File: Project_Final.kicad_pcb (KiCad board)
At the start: 2 copper layers, 73.5 x 111.5 mm, 54 parts, among them J1 Conn_01x02_Pin, J2 Conn_01x02_Pin, J3 Conn_01x02_Pin, J4 Conn_01x02_Pin, J5 Conn_01x02_Pin, Q1 2N3906, Q10 2N3906, Q11 2N3904, Q12 2N3906, Q13 2N3904, Q14 2N3904, Q15 2N3906, Q16 2N3906, Q17 BSP89, Q18 2N3904, Q19 2N3906, Q2 2N3906, Q20 2N3904, Q21 2N3904, Q22 2N3906, Q3 2N3906, Q4 2N3904, Q5 2N3904, Q6 2N3906, Q7 2N3906, Q8 2N3904, Q9 2N3906

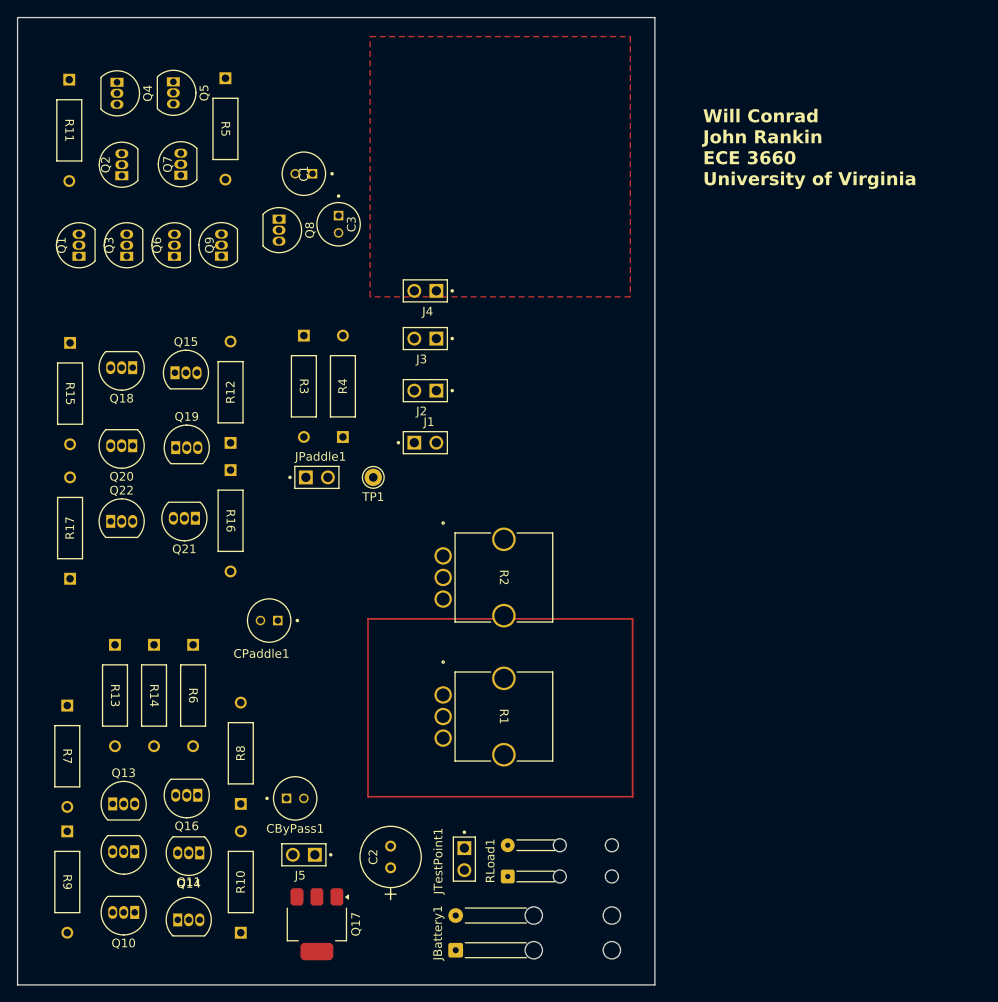
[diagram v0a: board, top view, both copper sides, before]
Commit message: finished layout
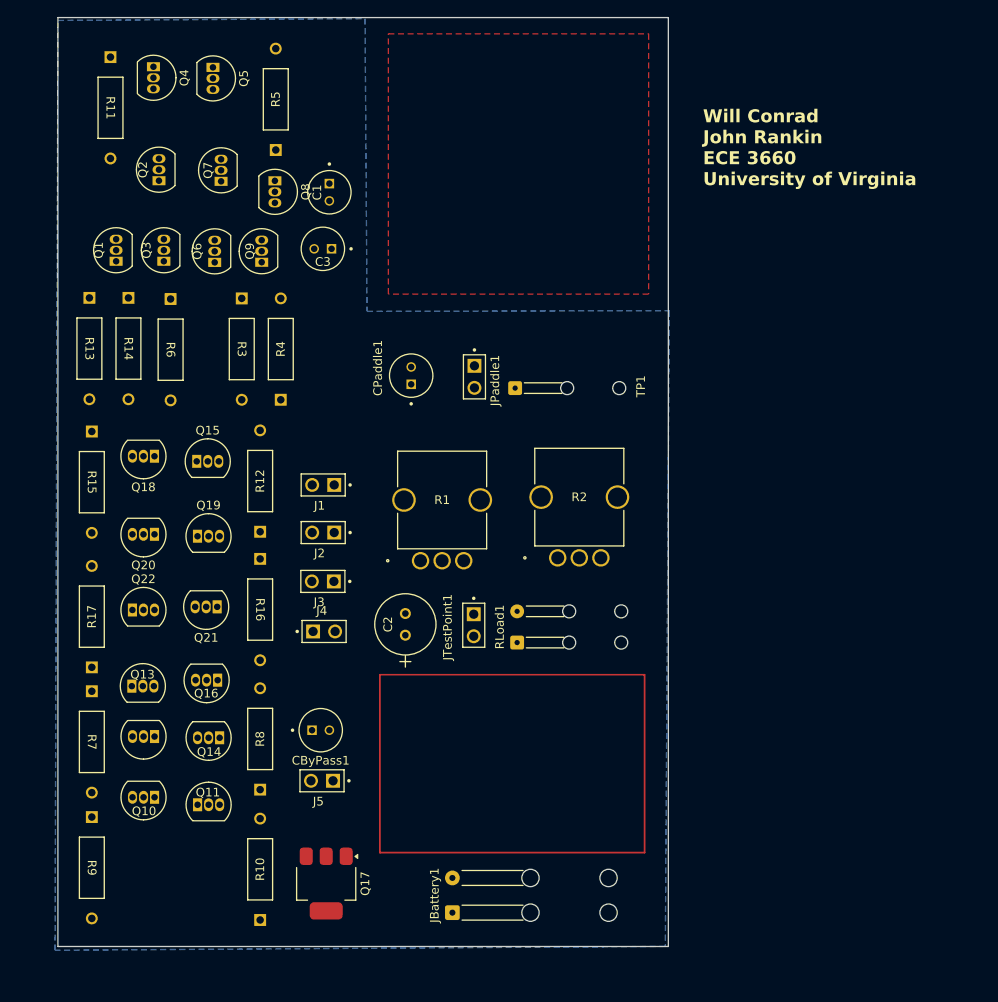
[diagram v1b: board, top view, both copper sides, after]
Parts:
- TP1: footprint Connector_Pin:Pin_D1.0mm_L10.0mm -> Library:Single_Relief
- moved J4 41.0 mm to (94.8, 87.3), turned to 0 degrees
- moved R13 40.1 mm to (67.8, 48.8)
- moved R14 40.1 mm to (72.3, 48.8)
- moved R6 39.9 mm to (77.1, 48.9)
- moved TP1 33.1 mm to (131.8, 59.0), turned to 90 degrees
- moved CPaddle1 32.6 mm to (104.9, 57.8), turned to 90 degrees
- moved J3 30.4 mm to (94.7, 81.5)
- moved JTestPoint1 27.0 mm to (112.1, 86.5)
- moved RLoad1 27.0 mm to (117.1, 88.5)
- moved C2 26.9 mm to (104.2, 87.7)
- moved JPaddle1 21.5 mm to (112.2, 57.9), turned to -90 degrees
- moved J2 20.2 mm to (94.7, 75.9)
- moved R1 15.7 mm to (105.9, 79.1), turned to 0 degrees
- moved Q13 13.8 mm to (72.7, 93.6)
- moved Q10 13.5 mm to (75.3, 106.4)
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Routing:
- added copper zone on B.Cu, net VEE
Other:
- board size 73.5 x 111.5 mm -> 70.4 x 107.1 mm
